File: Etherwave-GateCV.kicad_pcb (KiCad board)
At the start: 2 copper layers, 76 parts, among them J1 Etherwave Brd, J2 Volume CV, J3 Pitch CV, J4 Gate, Q1 PMP4501Y, Q2 PMBT3906, Q3 PMP4501Y, U1 LM13700, U2 CD4093, U3 CD4093, U4 CD4022, U5 TL072, U6 CD4016, U7 TL072

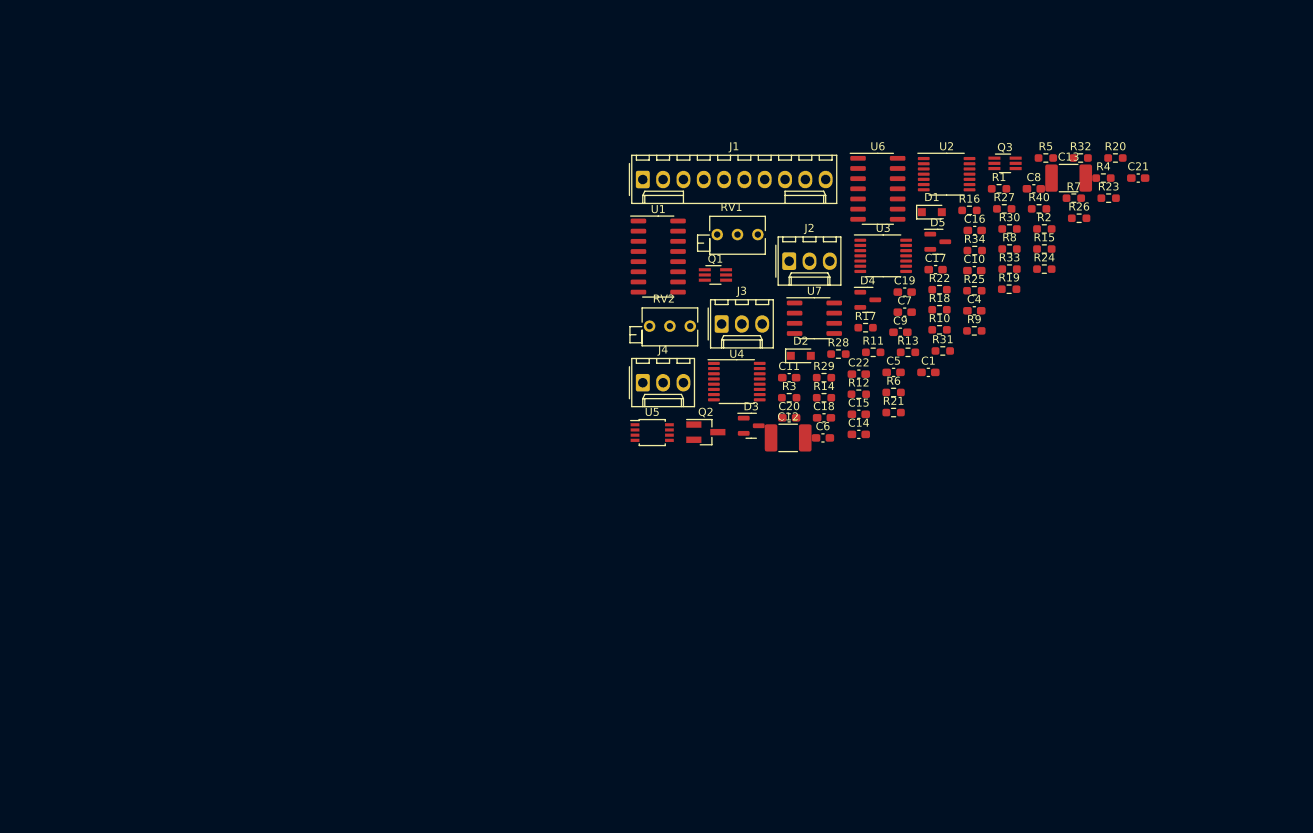
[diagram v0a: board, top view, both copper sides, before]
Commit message: about 40 % layout done
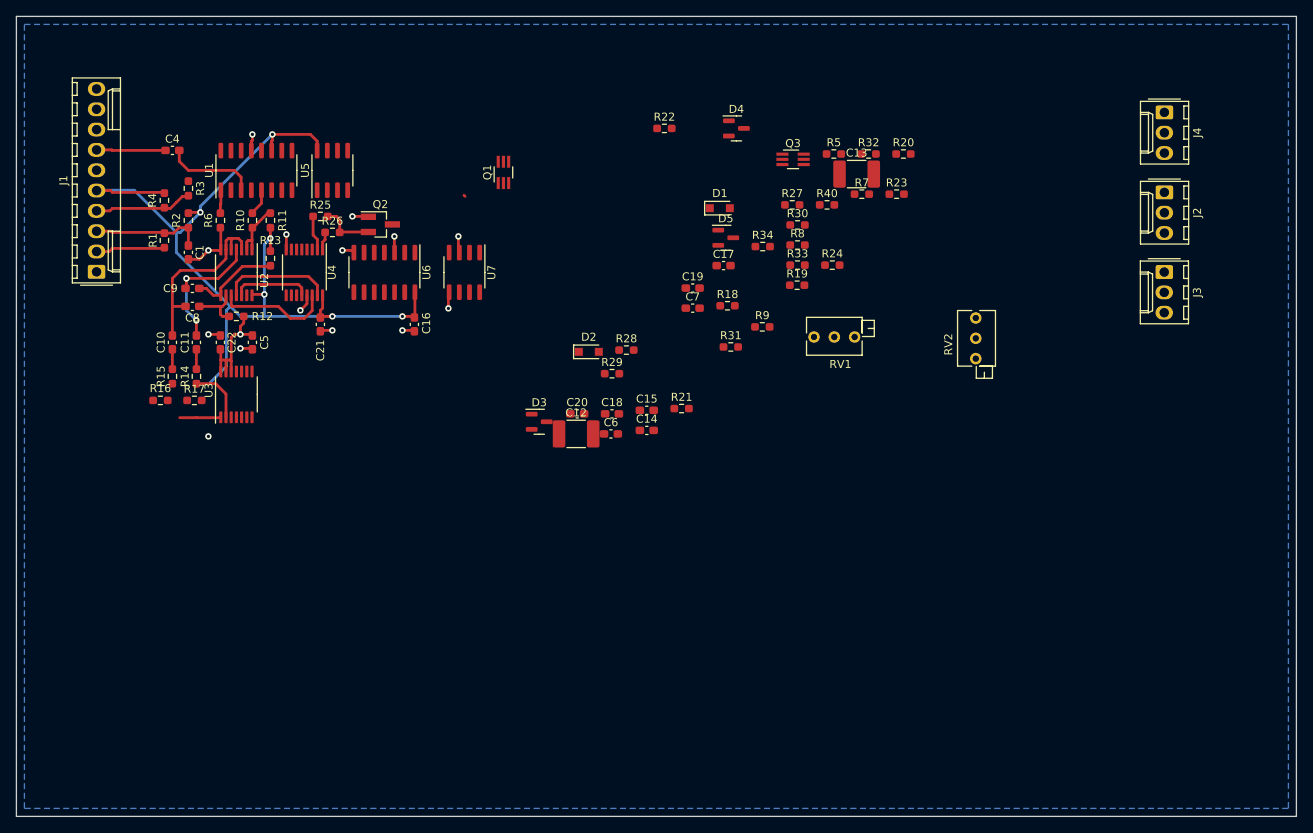
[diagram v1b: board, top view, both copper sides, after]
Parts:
- U5: footprint Package_SO:TSSOP-8_3x3mm_P0.65mm -> Package_SO:SOIC-8_3.9x4.9mm_P1.27mm
- moved R4 117.4 mm to (68.5, 73.0), turned to -90 degrees
- moved R15 110.1 mm to (69.5, 95.0), turned to 90 degrees
- moved R2 107.0 mm to (71.5, 75.5), turned to 90 degrees
- moved C8 106.2 mm to (72.0, 86.2), turned to 180 degrees
- moved R1 104.5 mm to (68.5, 78.0), turned to 90 degrees
- moved R16 103.9 mm to (68.0, 98.0), turned to 180 degrees
- moved C21 103.9 mm to (88.0, 88.5), turned to 90 degrees
- moved C4 102.2 mm to (69.5, 66.8)
- moved C10 100.6 mm to (69.5, 90.8), turned to 90 degrees
- moved C1 93.7 mm to (71.5, 79.5), turned to -90 degrees
- moved R26 93.4 mm to (89.5, 77.0)
- moved U2 89.6 mm to (77.5, 82.0), turned to -90 degrees
- moved C9 88.7 mm to (72.0, 84.0), turned to 180 degrees
- moved R10 87.0 mm to (79.5, 75.5), turned to -90 degrees
- moved R6 86.9 mm to (75.5, 75.5), turned to -90 degrees
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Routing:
- net +12V: track 0.00 -> 124.9 mm, vias 0 -> 8
- net GND: track 0.00 -> 31.0 mm, vias 0 -> 13
- net Net-(C10-Pad2): track 0.00 -> 23.4 mm
- net Net-(C11-Pad2): track 0.00 -> 17.5 mm, vias 0 -> 2
- net Net-(U2-Pad10): track 0.00 -> 14.4 mm
- net Net-(C1-Pad1): track 0.00 -> 14.2 mm
- net Net-(U2-Pad11): track 0.00 -> 13.8 mm
- net Net-(J1-Pad4): track 0.00 -> 12.3 mm
- net Net-(C4-Pad2): track 0.00 -> 11.5 mm
- net Net-(C9-Pad1): track 0.00 -> 11.3 mm
- net Net-(U2-Pad12): track 0.00 -> 9.78 mm
- net Net-(J1-Pad2): track 0.00 -> 8.68 mm
- net Net-(C4-Pad1): track 0.00 -> 8.64 mm
- net -12V: track 0.00 -> 8.61 mm
- net Net-(R10-Pad2): track 0.00 -> 7.44 mm
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- added copper zone on B.Cu, net GND
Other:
- board outline added: 160 x 100 mm
